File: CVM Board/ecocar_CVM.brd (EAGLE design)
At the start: 110.2 x 92.7 mm, 148 parts, among them U2 MAX3221CPWR

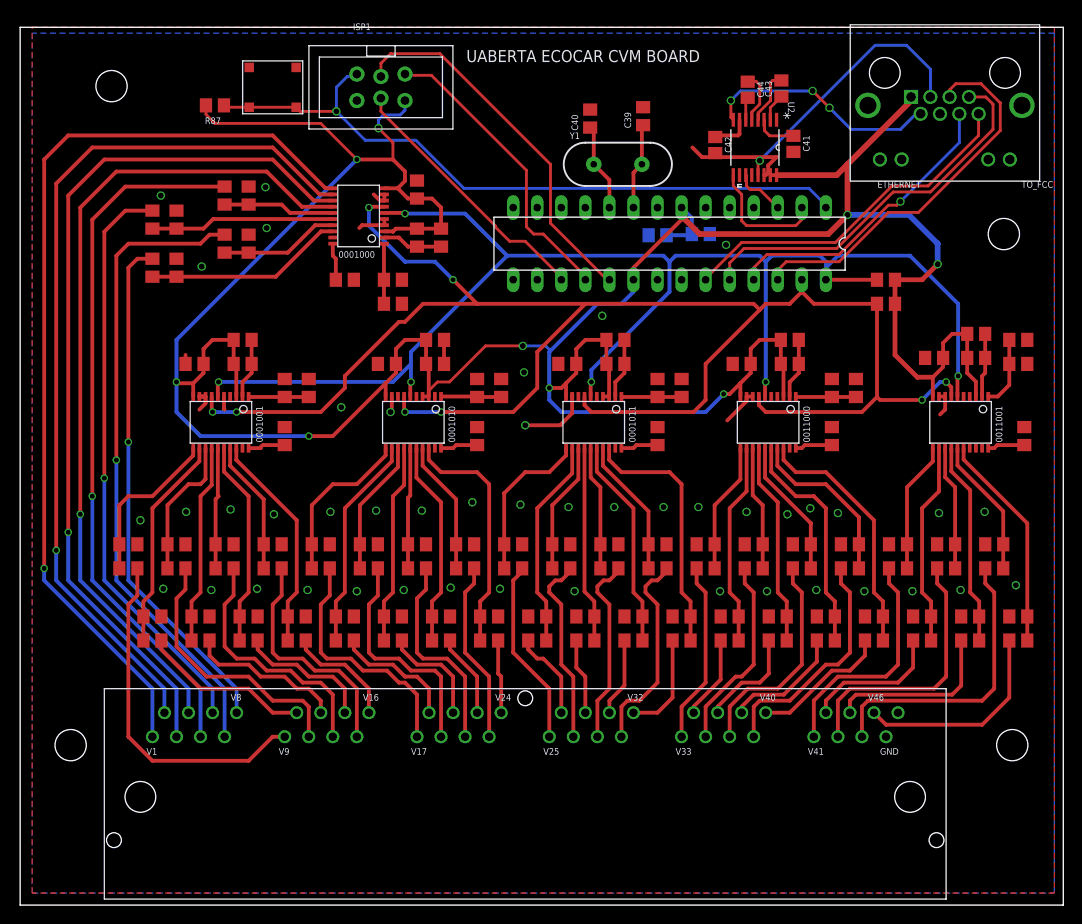
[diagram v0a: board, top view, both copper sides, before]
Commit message: update
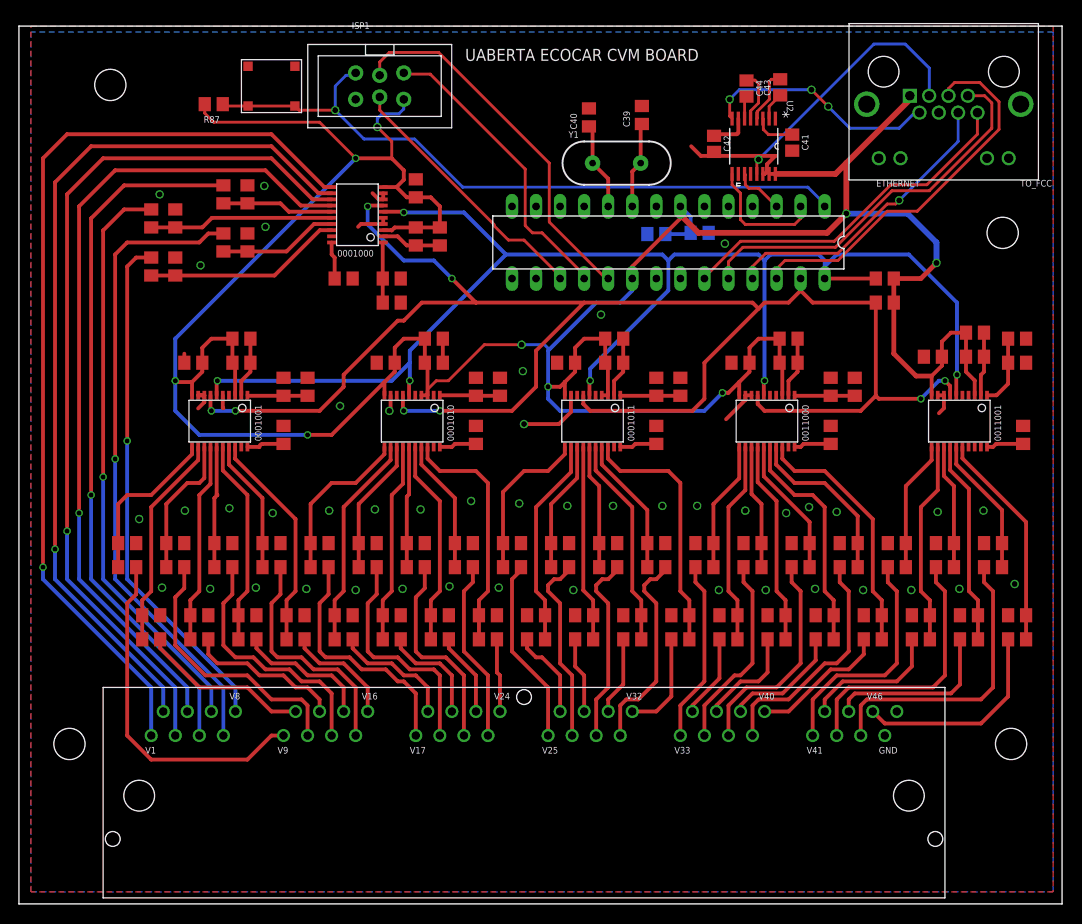
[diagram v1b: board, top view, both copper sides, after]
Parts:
- moved U2 0.18 mm to (77.6, 80.0)
- moved C20 0.18 mm to (69.8, 54.6)
- moved C25 0.18 mm to (85.7, 54.6)
- moved C30 0.18 mm to (85.7, 49.5)
- moved C4 0.18 mm to (39.4, 66.0)
- moved C40 0.18 mm to (60.2, 83.1)
- moved C6 0.18 mm to (34.3, 66.0)
- moved R1 0.18 mm to (24.1, 74.9)
- moved R44 0.18 mm to (64.8, 27.9)
- moved R48 0.18 mm to (69.8, 27.9)
- moved R57 0.18 mm to (82.5, 38.1)
- moved R58 0.18 mm to (82.5, 35.6)
- moved R61 0.18 mm to (87.6, 38.1)
- moved R62 0.18 mm to (87.6, 35.6)
- moved R73 0.18 mm to (105.4, 27.9)
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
